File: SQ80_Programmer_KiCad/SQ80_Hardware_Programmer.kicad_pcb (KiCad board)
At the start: 2 copper layers, 225 x 115 mm, 59 parts, among them J1 MIDI IN, J2 MIDI OUT/THRU, SW1 ARCH_MODE, SW2 GLITCH_TRIG, U1 MUX_1, U2 MUX_2, U3 6N138, U4 ER_OLEDM0.91_1x-I2C

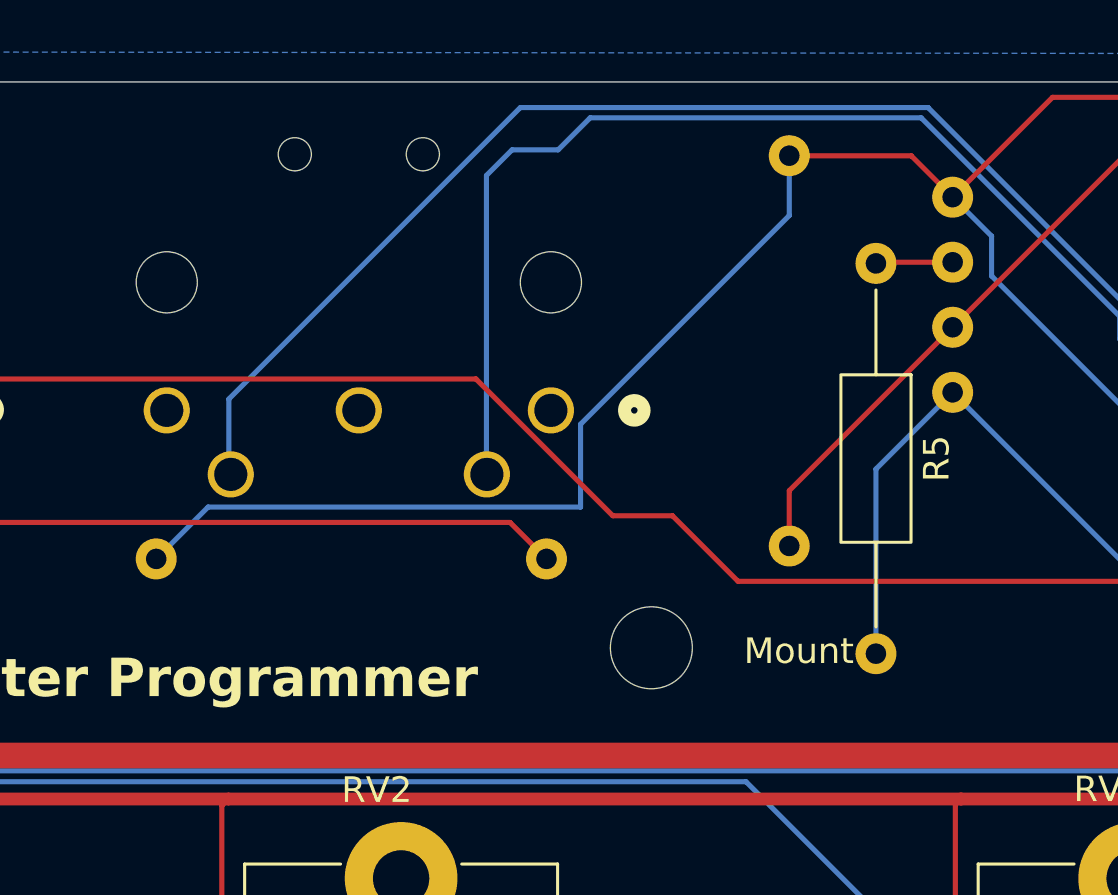
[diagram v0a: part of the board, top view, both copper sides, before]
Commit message: README Edits
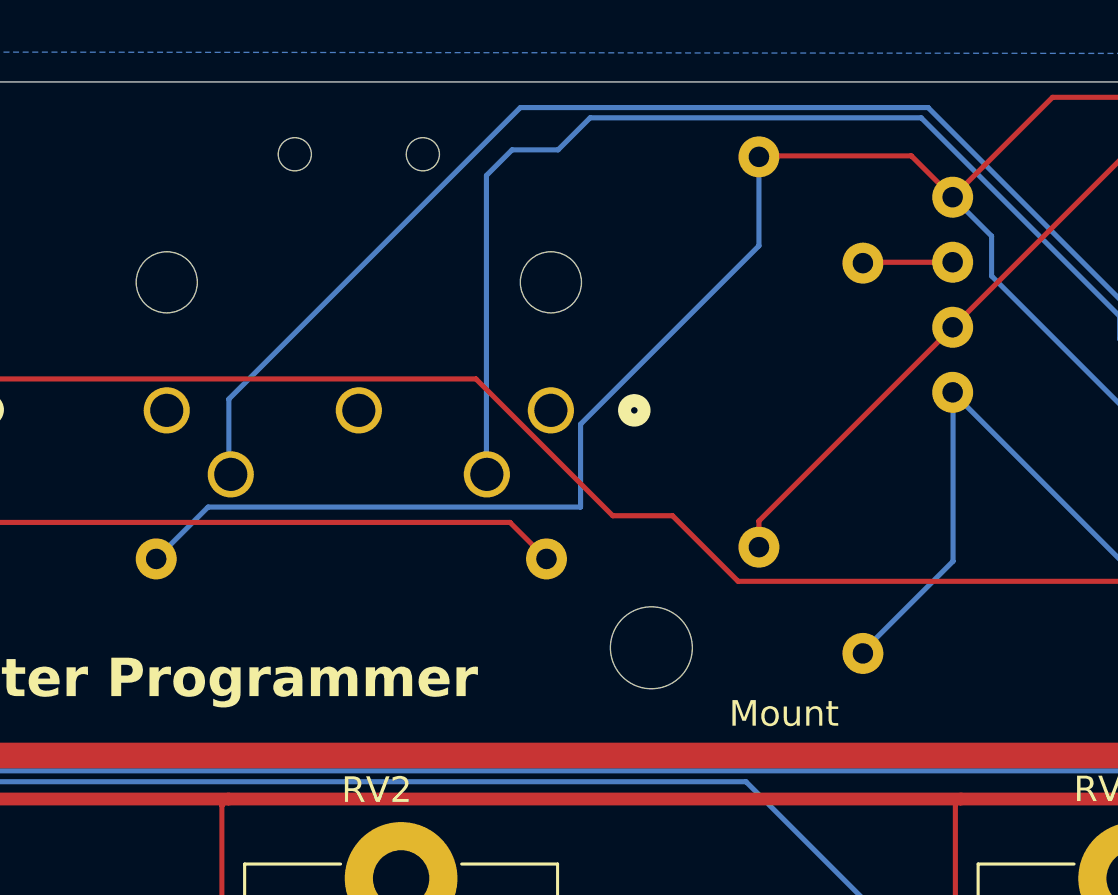
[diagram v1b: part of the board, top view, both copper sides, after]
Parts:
- R5: moved to B.Cu
- moved R4 1.19 mm to (91.9, 36.6)
- moved R5 0.51 mm to (96.0, 40.8)
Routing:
- net +5V: track 1501.8 -> 1502.4 mm
- net /MIDI_RX: track 139.5 -> 140.0 mm
